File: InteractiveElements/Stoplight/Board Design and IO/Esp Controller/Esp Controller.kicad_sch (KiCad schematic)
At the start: 5 parts, among them J1 RJ45, J2 RJ45, J3 RJ45, J4 RJ45, U2 ESP32-DevKitC

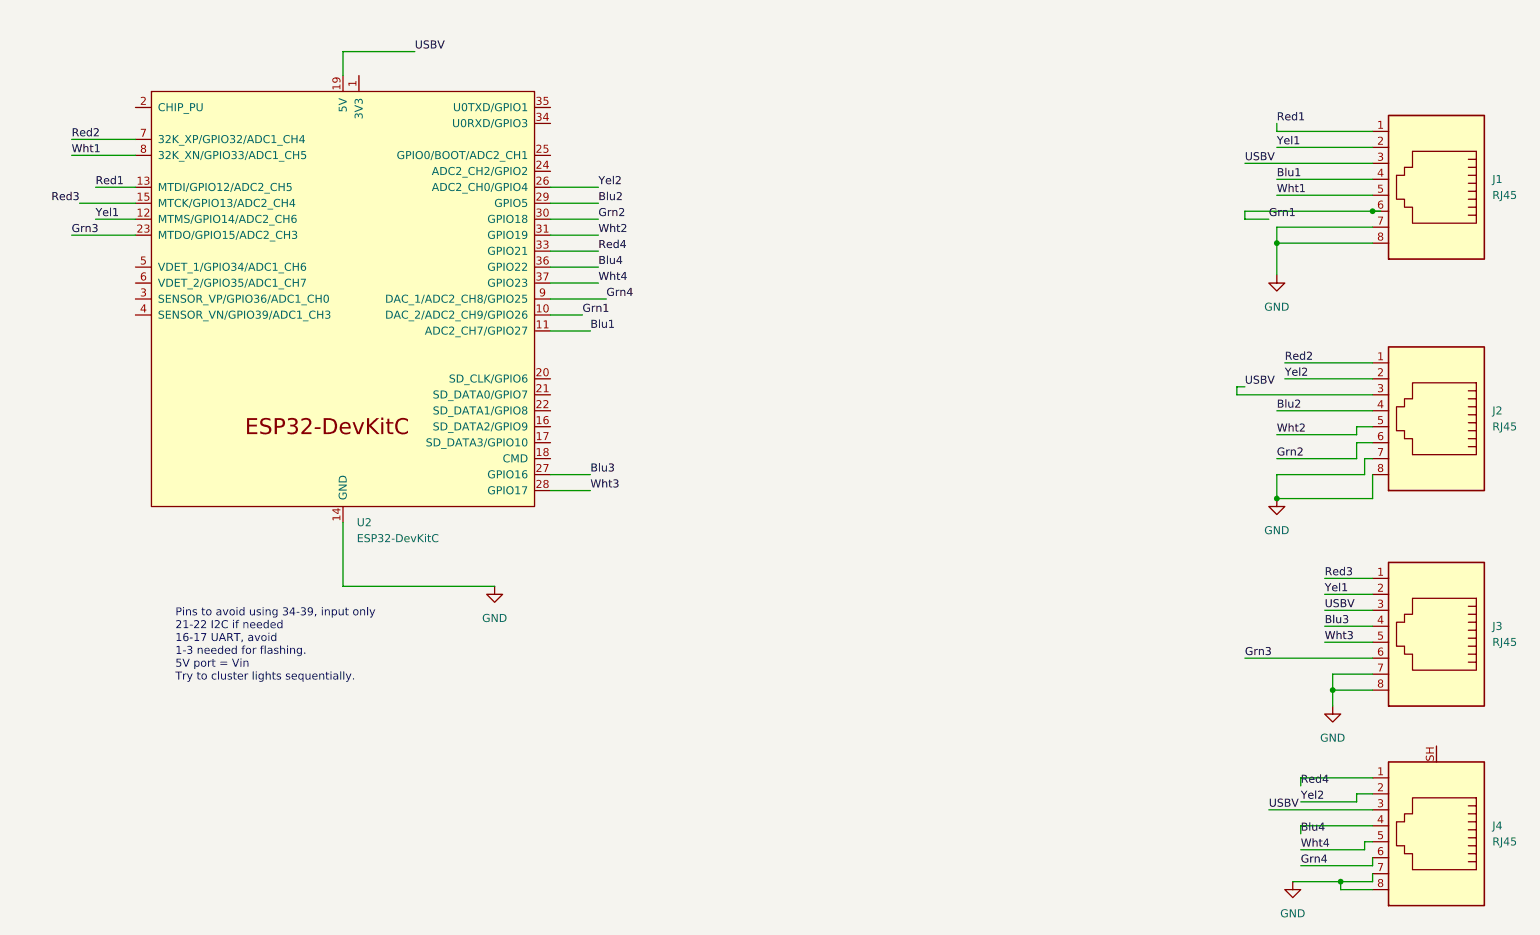
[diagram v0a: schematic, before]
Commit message: updated schematic
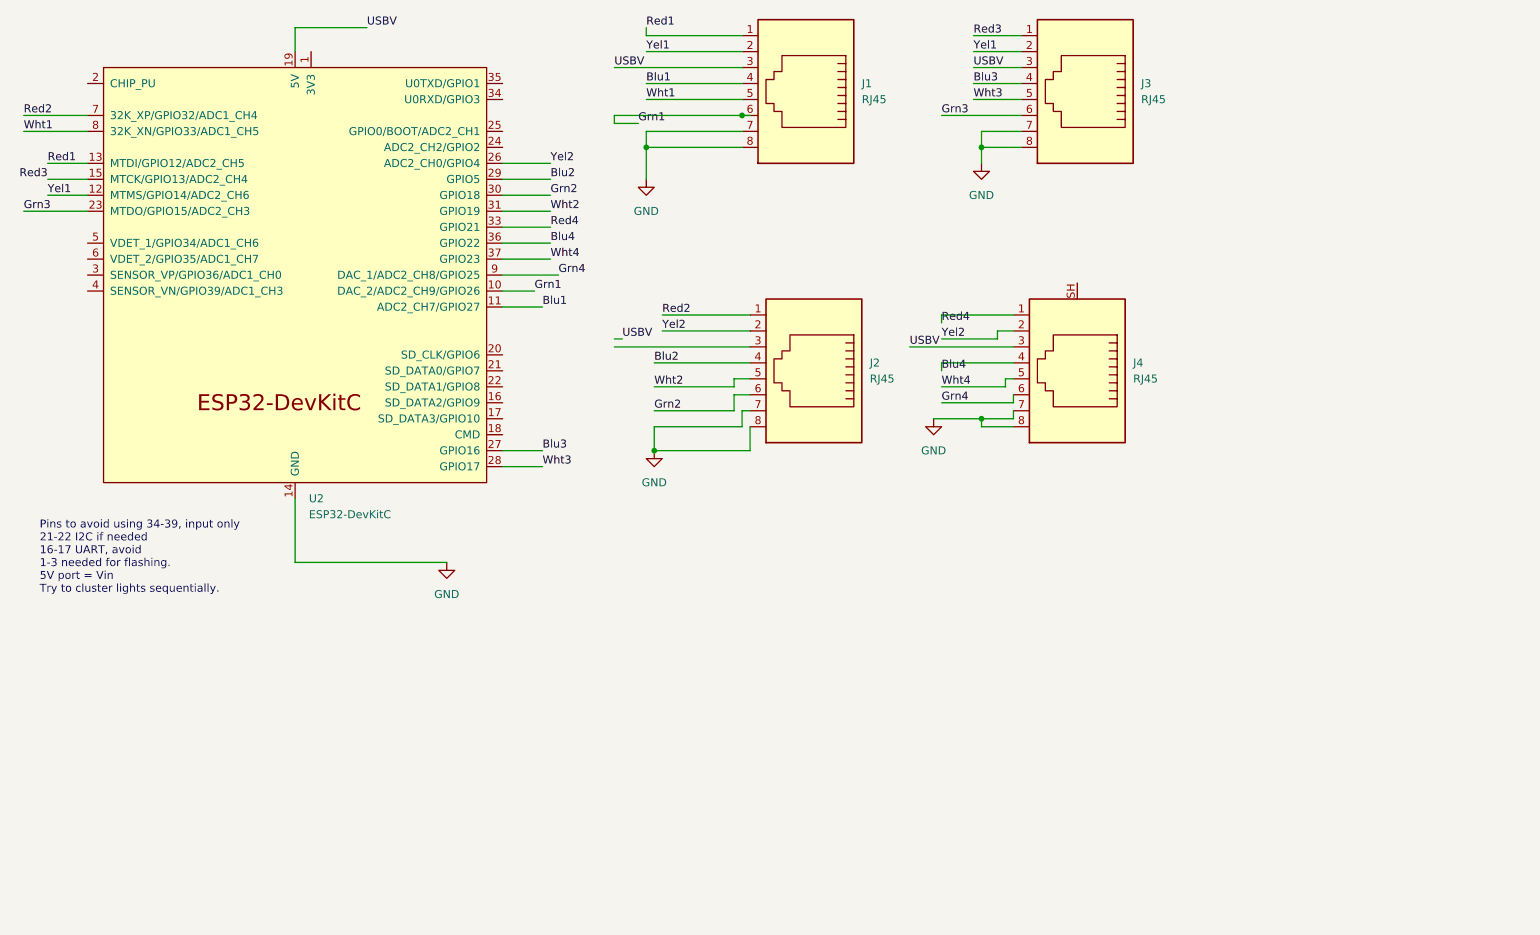
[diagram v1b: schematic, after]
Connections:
- net USBV: no longer J2.3
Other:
- title: (none) -> Interactive Element Receiver Board
- moved on the sheet: J1, J2, J3, J4, U2
